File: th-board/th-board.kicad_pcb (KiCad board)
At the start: 2 copper layers, 59.5 x 48.5 mm, 23 parts, among them J1 Conn_01x02, J2 Conn_01x04, U1 ESP-12F, U2 DHT11, U3 SPX3819M5-L

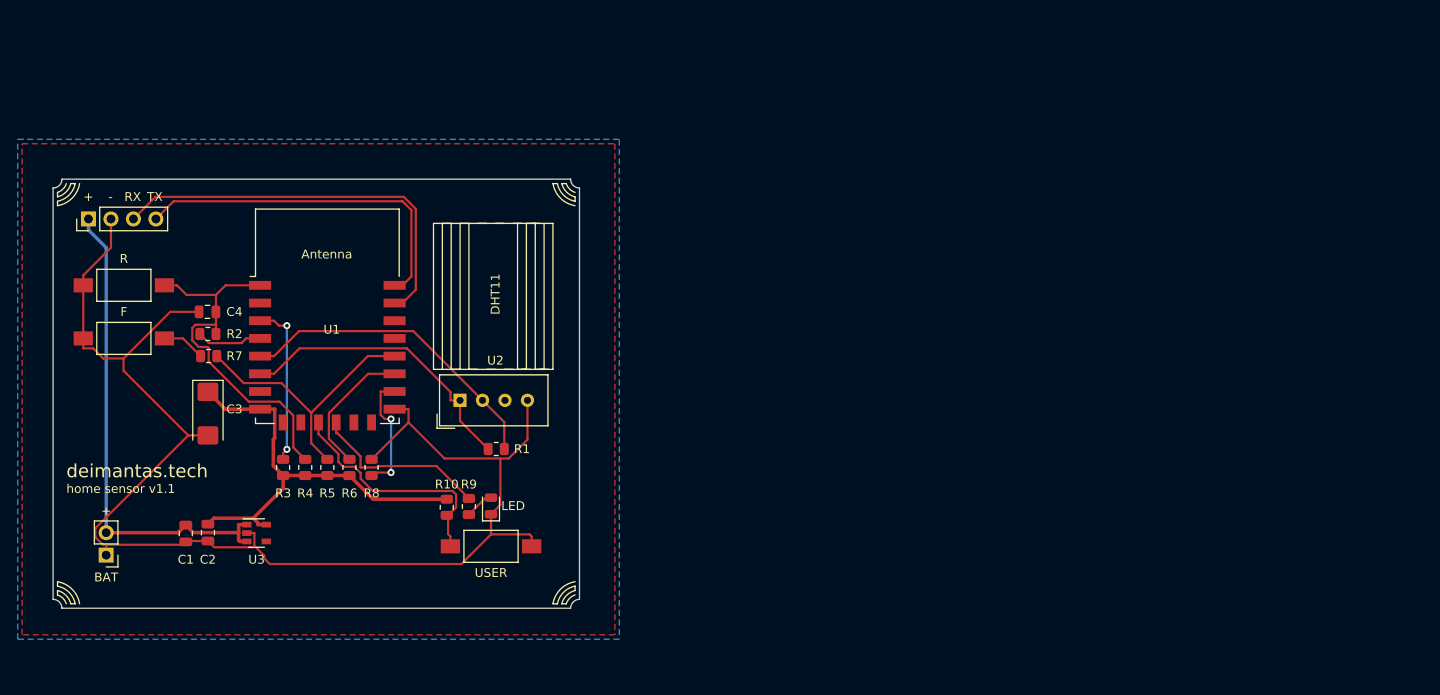
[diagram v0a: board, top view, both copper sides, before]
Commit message: PCB: new board
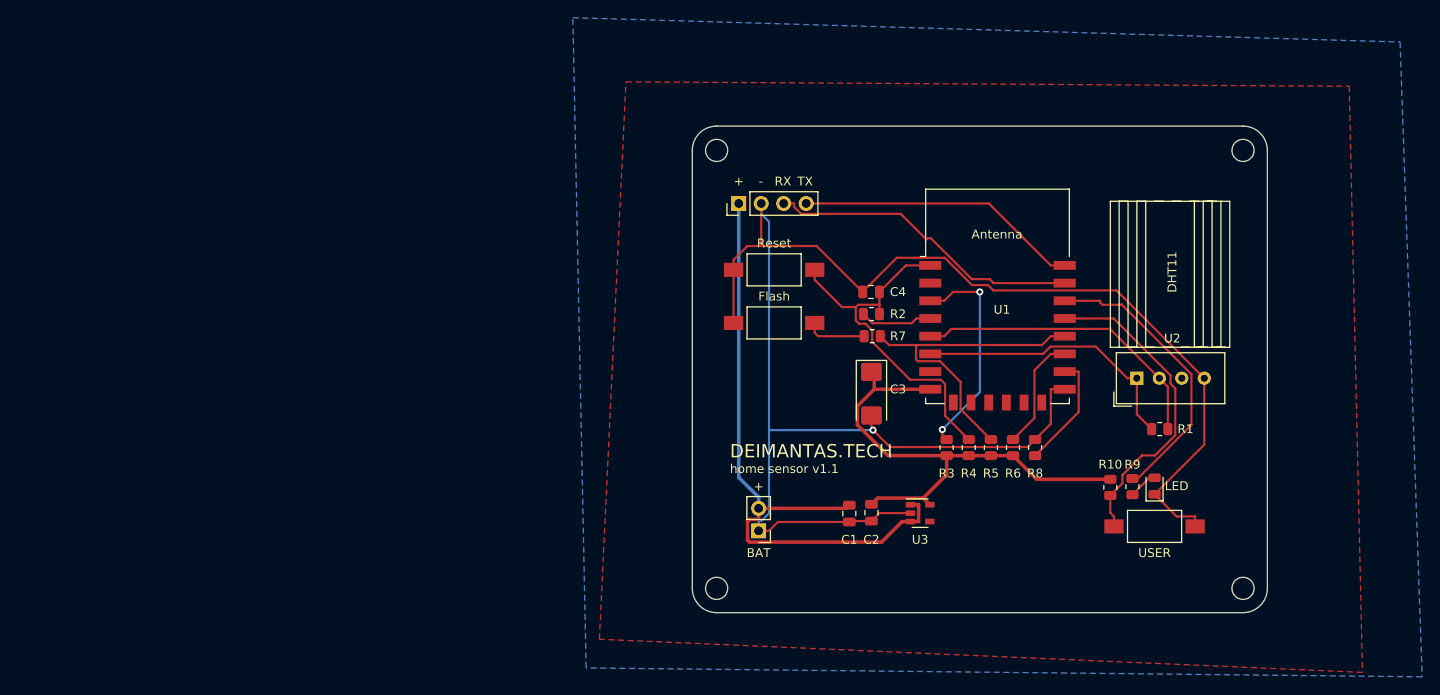
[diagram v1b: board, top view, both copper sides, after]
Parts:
- moved U2 76.5 mm to (241.5, 97.5)
- moved U1 75.8 mm to (225.8, 88.2)
- moved C1 75.0 mm to (209.0, 112.8)
- moved C2 75.0 mm to (211.5, 112.7)
- moved C3 75.0 mm to (211.5, 99.2)
- moved C4 75.0 mm to (211.4, 87.8)
- moved D1 75.0 mm to (243.5, 109.7)
- moved R1 75.0 mm to (244.1, 103.2)
- moved R10 75.0 mm to (241.0, 109.8)
- moved R2 75.0 mm to (211.5, 90.2)
- moved R3 75.0 mm to (220.0, 105.3)
- moved R4 75.0 mm to (222.5, 105.3)
- moved R5 75.0 mm to (225.0, 105.3)
- moved R6 75.0 mm to (227.5, 105.3)
- moved R7 75.0 mm to (211.6, 92.8)
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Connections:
- R10 pad 2: Net-(R10-Pad2) -> USER_LED
- R9 pad 1: Net-(R9-Pad1) -> USER_BUTTON
- SW_User2 pad 2: Net-(R9-Pad1) -> USER_BUTTON
- U1 pad 11: Net-(R9-Pad1) -> Net-(U1-Pad11)
- U1 pad 12: Net-(R10-Pad2) -> Net-(U1-Pad12)
- U1 pad 19: Net-(U1-Pad19) -> USER_BUTTON
- U1 pad 20: Net-(U1-Pad20) -> USER_LED
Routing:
- net GND: track 157.2 -> 194.4 mm, vias 0 -> 1
- net USER_BUTTON: track 0.00 -> 36.0 mm
- net USER_LED: track 0.00 -> 32.8 mm
- net Net-(R9-Pad1): track 27.1 -> 0.00 mm
- net Net-(R10-Pad2): track 20.1 -> 0.00 mm
- net Net-(C1-Pad1): track 55.6 -> 73.7 mm
- net RX: track 45.7 -> 35.8 mm
- net VCC: track 49.5 -> 57.5 mm
- net TX: track 39.9 -> 32.1 mm
- net Net-(R3-Pad2): track 18.6 -> 24.7 mm
- net Net-(R5-Pad2): track 31.4 -> 37.3 mm
- net Net-(R6-Pad2): track 15.5 -> 13.0 mm
- net DHT11_VCC: track 33.6 -> 31.6 mm
- net Net-(R7-Pad2): track 4.91 -> 6.87 mm
- net DHT11_IO: track 36.1 -> 34.7 mm
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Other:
- board size 59.5 x 48.5 mm -> 65 x 55 mm
- board text added: "DEIMANTAS.TECH"
- board text added: "Flash"
- board text added: "Reset"
- board text removed: "F"
- board text removed: "R"
- board text removed: "deimantas.tech"
